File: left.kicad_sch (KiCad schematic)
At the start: 65 parts, among them J3 LEFT, Q1 IRF540N, Q2 IRF540N, Q3 IRF540N, Q4 IRF540N, U1 TL072, U2 TL072, U4 LT1016, U5 IR2184, U6 IR2184

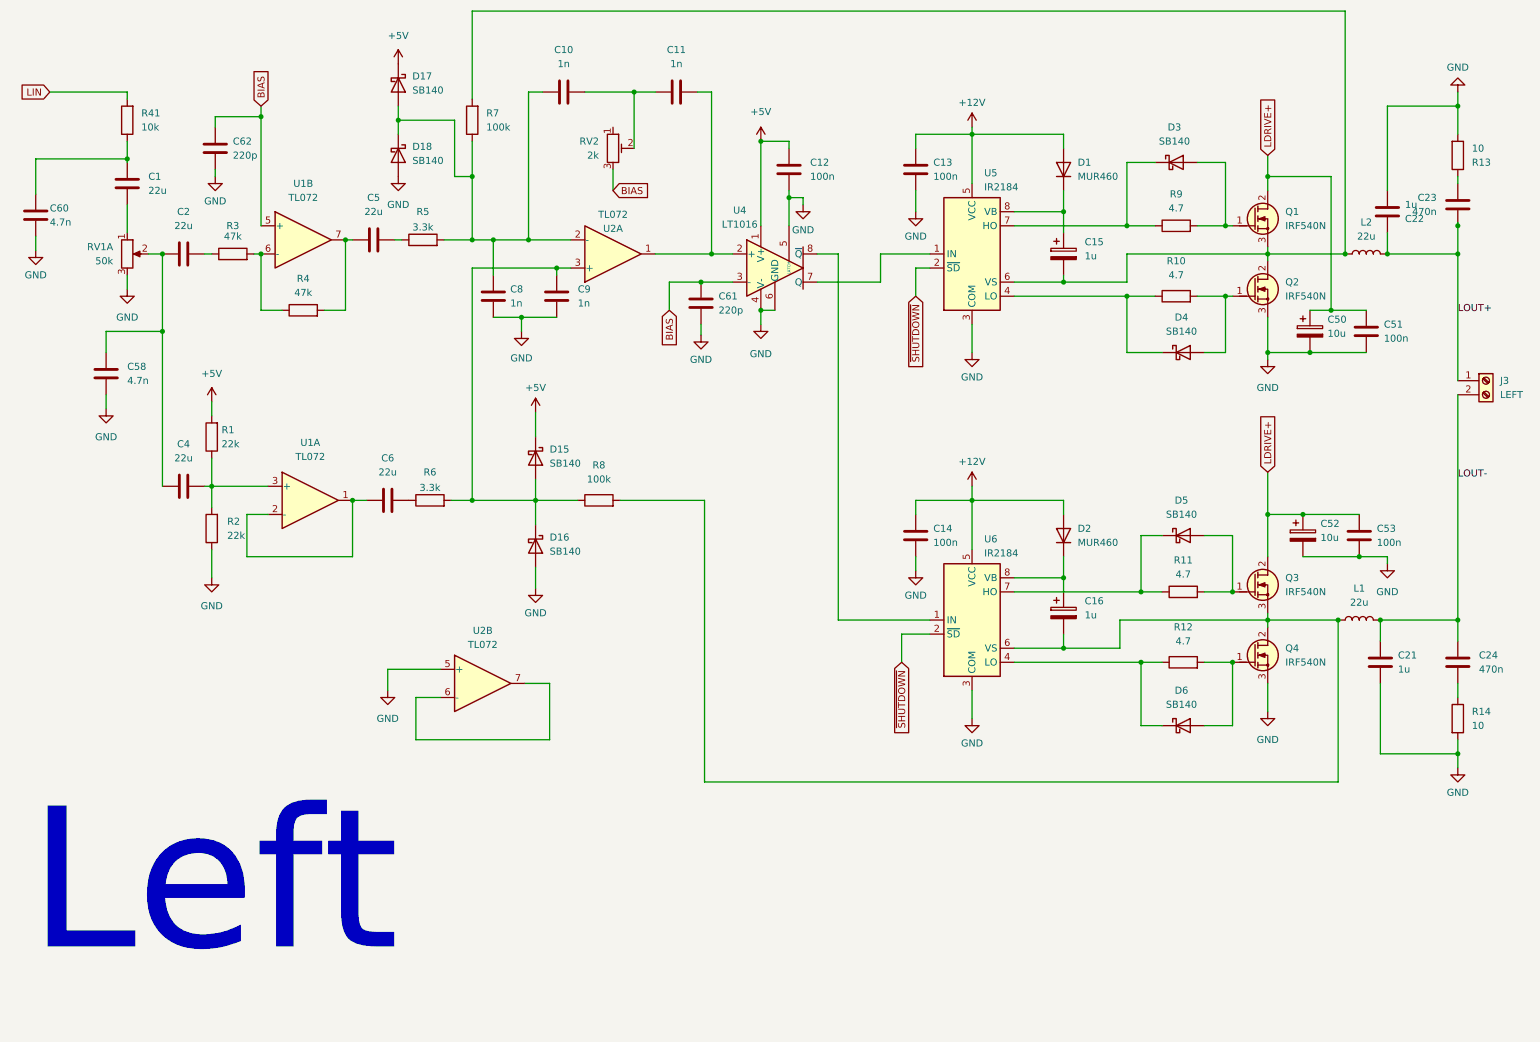
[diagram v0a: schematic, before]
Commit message: WIP
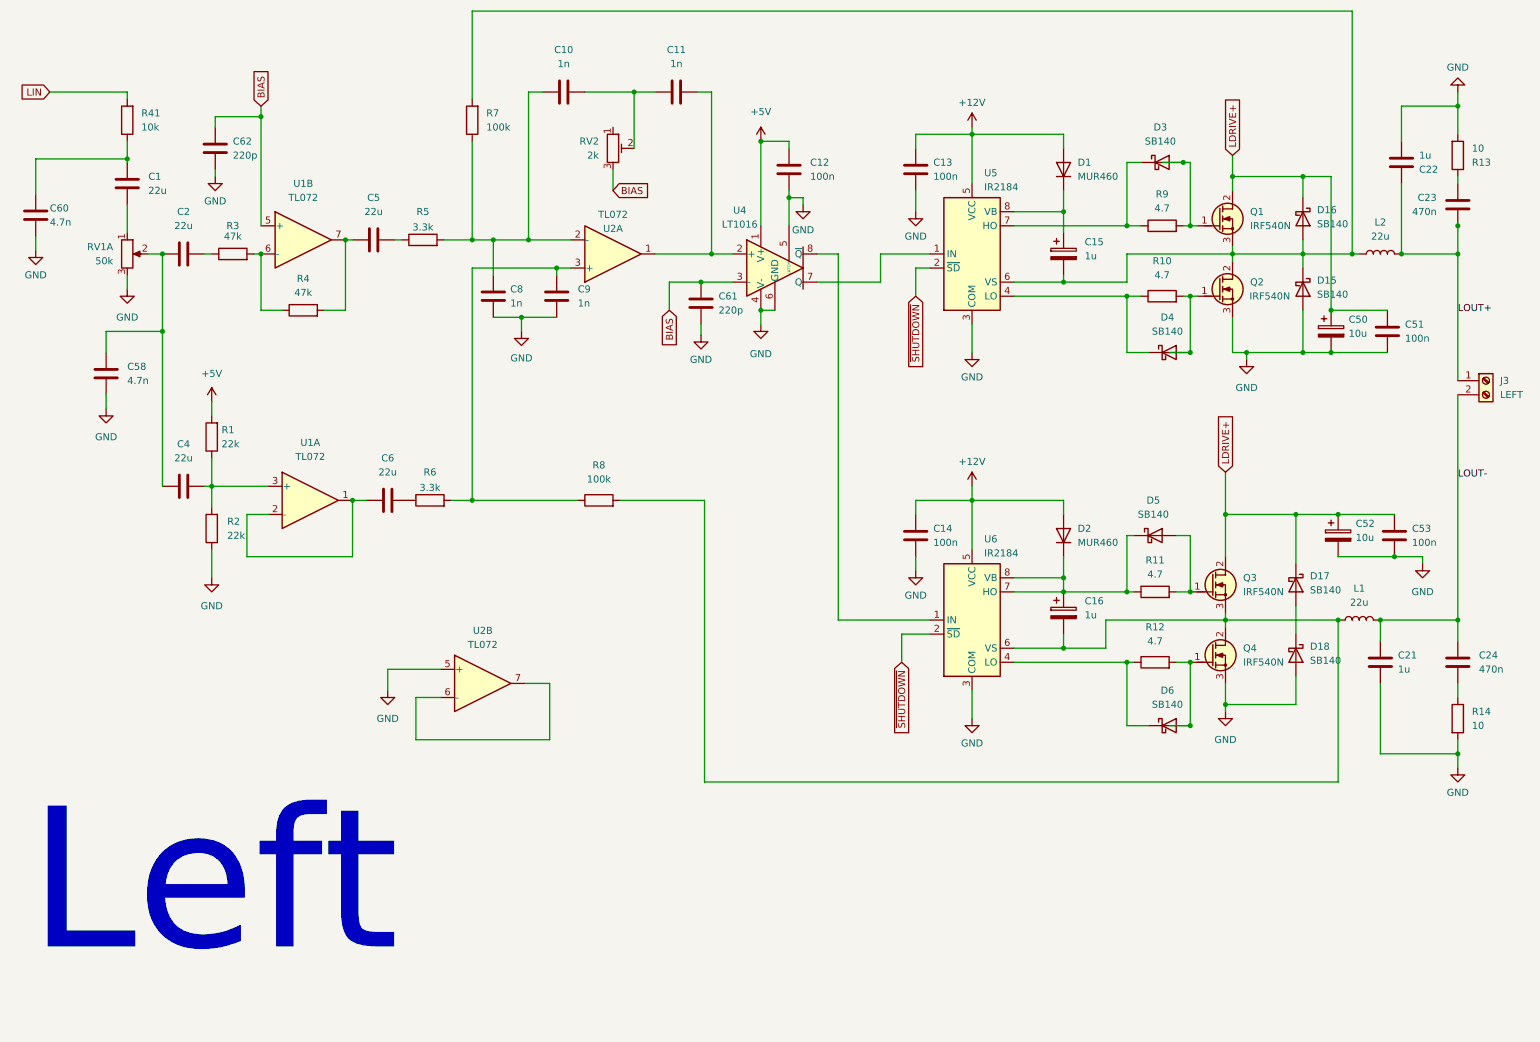
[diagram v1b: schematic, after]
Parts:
- C1, C2, C4, C5, C6: footprint Capacitor_THT:CP_Radial_D8.0mm_P3.50mm -> Capacitor_THT:CP_Radial_D4.0mm_P1.50mm
- U1, U2, U4, U5, U6: footprint PCM_Package_DIP_AKL:DIP-8_W7.62mm -> Package_DIP:DIP-8_W7.62mm
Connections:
- net +5V: no longer D15.1 (K), D17.1 (K)
- net GND: now also D15.2 (A); no longer D16.2 (A)
- net LDRIVE+: now also D16.1 (K), D17.1 (K)
- net at C15.2, L2.1, Q1.3 (S)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: now also D15.1 (K), D16.2 (A)
- net at C16.1, D2.1 (K), U6.8 (VB): now also D5.1 (K), R11.1, U6.7 (HO)
- net at C10.1, C8.1, R5.2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: no longer D17.2 (A), D18.1 (K)
- net at C9.1, R6.2, R8.1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: no longer D15.2 (A), D16.1 (K)
- new net: D17.2 (A), D18.1 (K)
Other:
- moved on the sheet: C22, C50, C51, C52, C53, D3, D4, D5, D6, L2, Q1, Q2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
